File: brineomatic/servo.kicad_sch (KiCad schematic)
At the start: 8 parts, among them J8 SERVOS, U2 XL1509-5.0

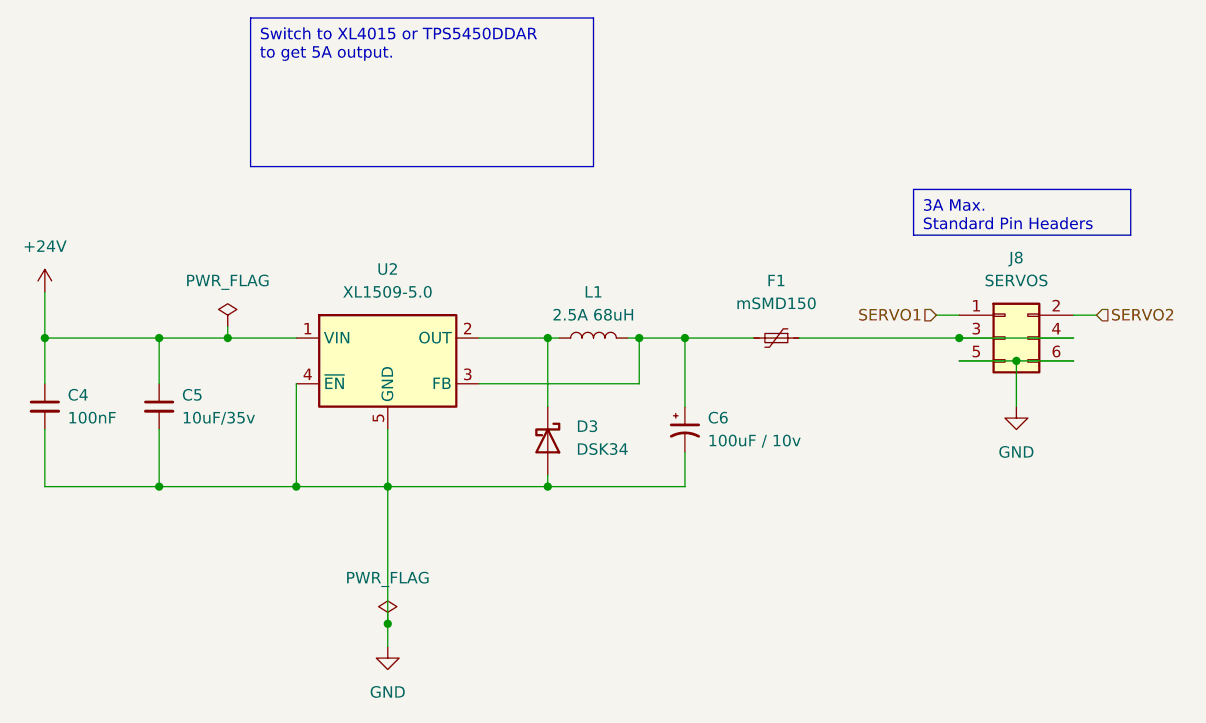
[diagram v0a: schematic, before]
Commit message: kicad v9 and updated todo.
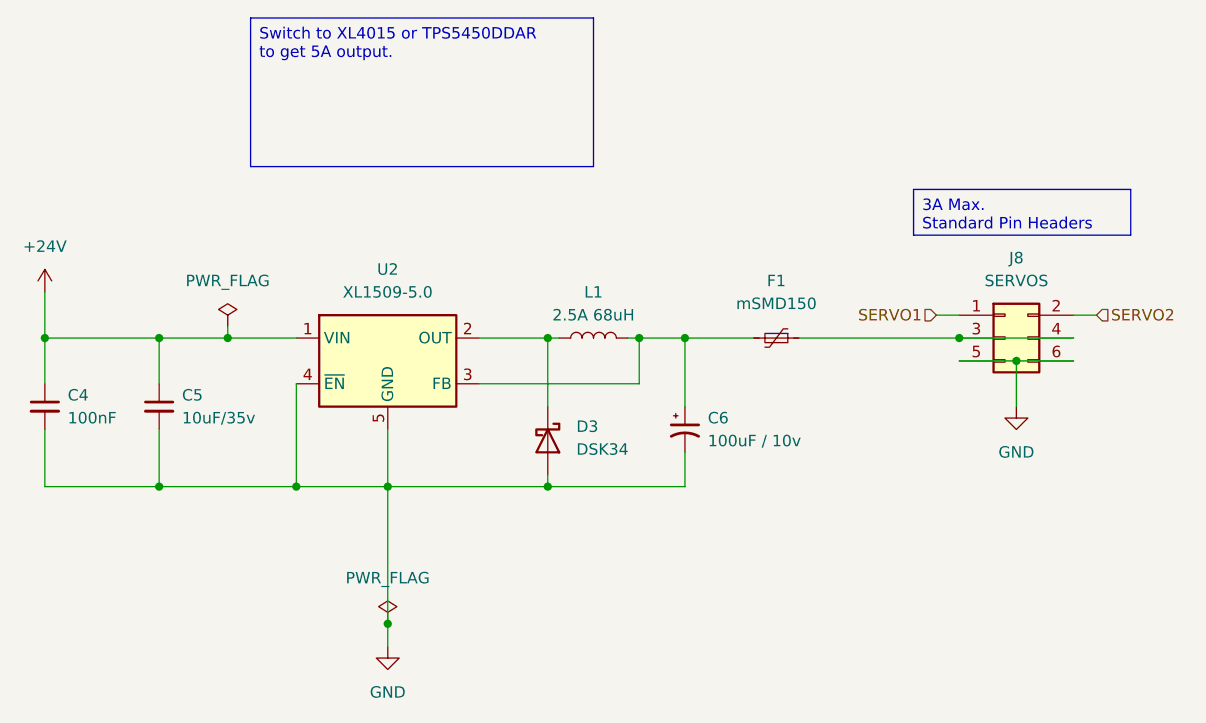
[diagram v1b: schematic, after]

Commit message: worked on schematic and layout a bit more.
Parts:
- C4: footprint Capacitor_SMD:C_0805_2012Metric_Pad1.18x1.45mm_HandSolder -> Capacitor_SMD:C_0603_1608Metric
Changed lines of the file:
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@@
 			)
 		)
-		(property "Footprint" "Capacitor_SMD:C_0805_2012Metric_Pad1.18x1.45mm_HandSolder"
+		(property "Footprint" "Capacitor_SMD:C_0603_1608Metric"
 			(at 67.31 134.62 0)
 			(effects
